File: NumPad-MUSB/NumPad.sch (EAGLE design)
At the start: 102 parts, among them IC1 74AC138N, IC2 74AC00N, J2 J

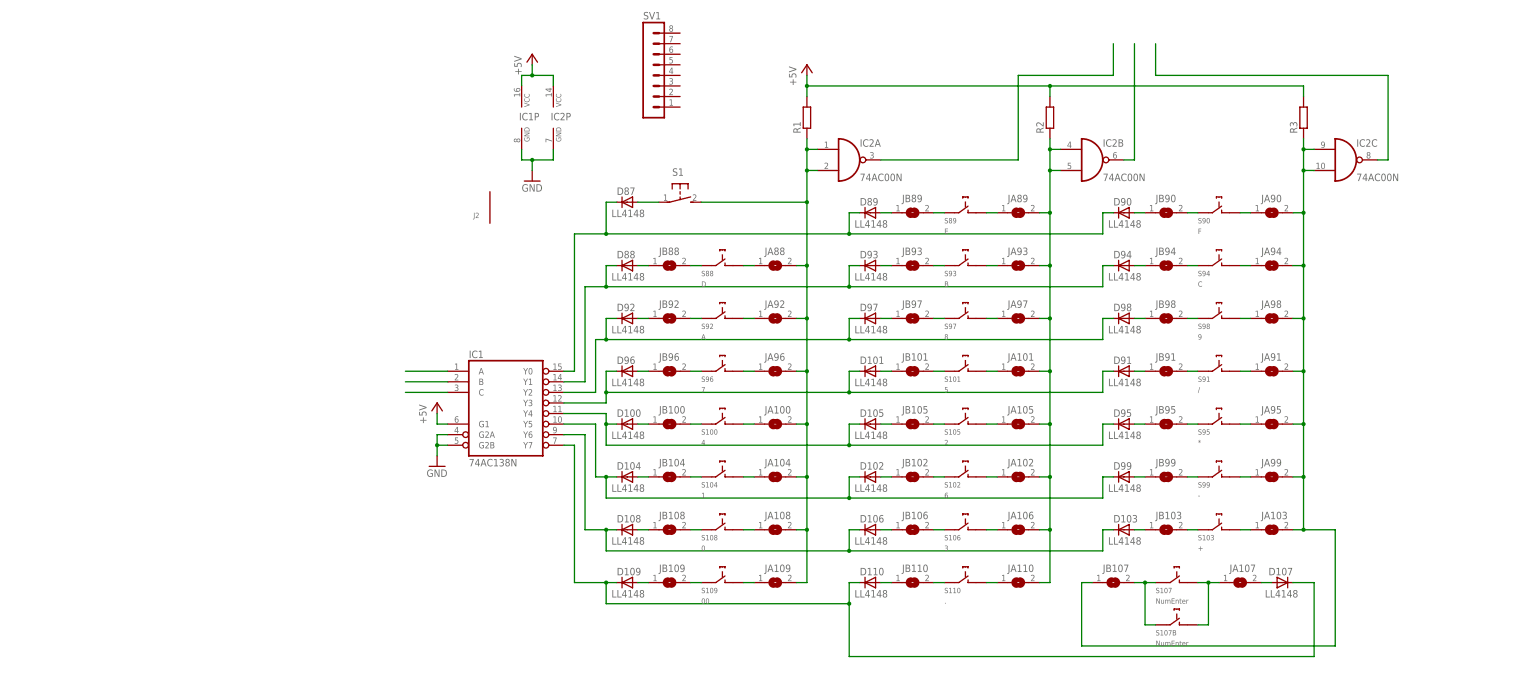
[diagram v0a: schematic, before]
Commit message: pcb np
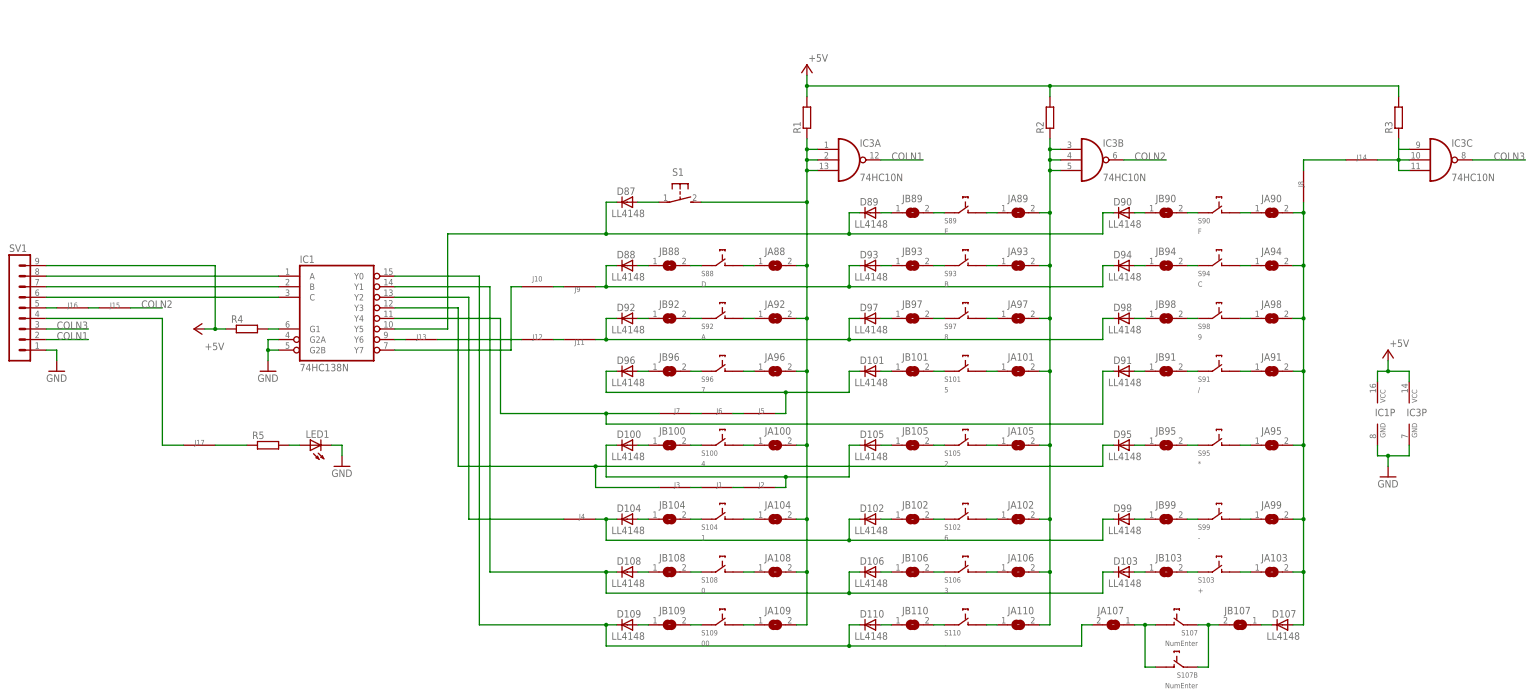
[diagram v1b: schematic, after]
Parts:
- removed IC2: 74AC00N, 74xx-eu:74AC00N
- added IC3: 74HC10N, detali:74HC10N
- added J1, J10, J11, J12, J13, J14, J15, J16, J17, J3, J4, J5, J6, J7, J8, J9: J, detali:J
- added LED1: (no value), detali:LED5MM
- added R4, R5: (no value), rcl:R-EU_R1206W
- IC1: value 74AC138N -> 74HC138N; device 74xx-eu:74AC138N -> detali:74HC138N
- R1, R2, R3: device rcl:R-EU_R0805 -> rcl:R-EU_R1206W
- S1: device switch-omron:31-XX -> detali:31-XX
- SV1: device con-lstb:MA08-1 -> detali:MA09-1
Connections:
- new net COLN1: IC3A.O, SV1.2
- new net COLN2: IC3B.O, J15.P$1
- new net COLN3: IC3C.O, SV1.3
- new net N$15: J5.P$2, J6.P$1
- new net N$17: IC3C.I0, IC3C.I1, IC3C.I2, J14.P$1, R3.1
- new net N$18: IC1A.Y7, J10.P$1
- new net N$19: J10.P$2, J9.P$1
- new net N$20: J11.P$1, J12.P$1
- new net N$21: J12.P$2, J13.P$1
- new net N$23: IC1A.Y6, J13.P$2
- new net N$24: IC1A.G1, R4.2
- new net N$26: J14.P$2, J8.P$1
- new net N$27: LED1.A, R5.2
- new net N$28: J16.P$2, SV1.5
- new net N$29: J15.P$2, J16.P$1
- new net N$3: D107.C, JB107.1
- new net N$30: J17.P$2, SV1.4
- new net N$31: J17.P$1, R5.1
- new net N$4: J1.P$2, J3.P$1
- new net N$5: J1.P$1, J2.P$2
- net +5V: now also IC3P.VCC, R4.1, SV1.9; no longer IC1A.G1, IC2P.VCC
- net GND: now also IC3P.GND, LED1.C, SV1.1; no longer IC2P.GND
- net N$1: now also J11.P$2; no longer IC1A.Y2
- net N$10: now also IC1A.C, SV1.6; no longer IC1A.A
- net N$11: now also IC1A.Y2, J4.P$2; no longer IC2C.O
- net N$12: now also D101.C, D96.C, J5.P$1; no longer IC2B.O
- net N$13: now also J6.P$2, J7.P$1; no longer IC2A.O
- net N$14: now also IC3A.I0, IC3A.I1, IC3A.I2; no longer IC2A.I0, IC2A.I1
- net N$16: now also J9.P$2; no longer IC1A.Y1
- net N$2: now also D100.C, D105.C, J2.P$1; no longer D107.A, JA107.2
- net N$22: now also D107.A, J8.P$2; no longer IC2C.I0, IC2C.I1, JB107.1, R3.1
- net N$33: now also IC1A.Y5; no longer IC1A.Y0
- net N$34: now also IC1A.Y4, J7.P$2; no longer D101.C, D96.C, IC1A.Y3
- net N$35: now also IC1A.Y3, J3.P$2; no longer D100.C, D105.C, IC1A.Y4
- net N$36: now also IC1A.Y1; no longer IC1A.Y6
- net N$6: now also IC1A.A, SV1.8; no longer IC1A.C
- net N$7: now also IC3B.I0, IC3B.I1, IC3B.I2; no longer IC2B.I0, IC2B.I1
- net N$8: now also SV1.7
- net N$9: now also J4.P$1; no longer IC1A.Y5
- net SCK: now also IC1A.Y0, JA107.2; no longer D107.C, IC1A.Y7
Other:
- moved on the sheet: D100, D102, D103, D104, D105, D106, D107, D108, D109, D110, D95, D99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
